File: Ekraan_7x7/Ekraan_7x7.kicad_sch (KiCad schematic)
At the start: 37 parts, among them IC1 74HC595PW-Q100,118, IC10 1EDN7550BXTSA1, IC11 1EDN7550BXTSA1, IC3 1EDN7550BXTSA1, IC6 1EDN7550BXTSA1, IC7 1EDN7550BXTSA1, IC8 1EDN7550BXTSA1, IC9 1EDN7550BXTSA1, U1 1EDN7550BXTSA1

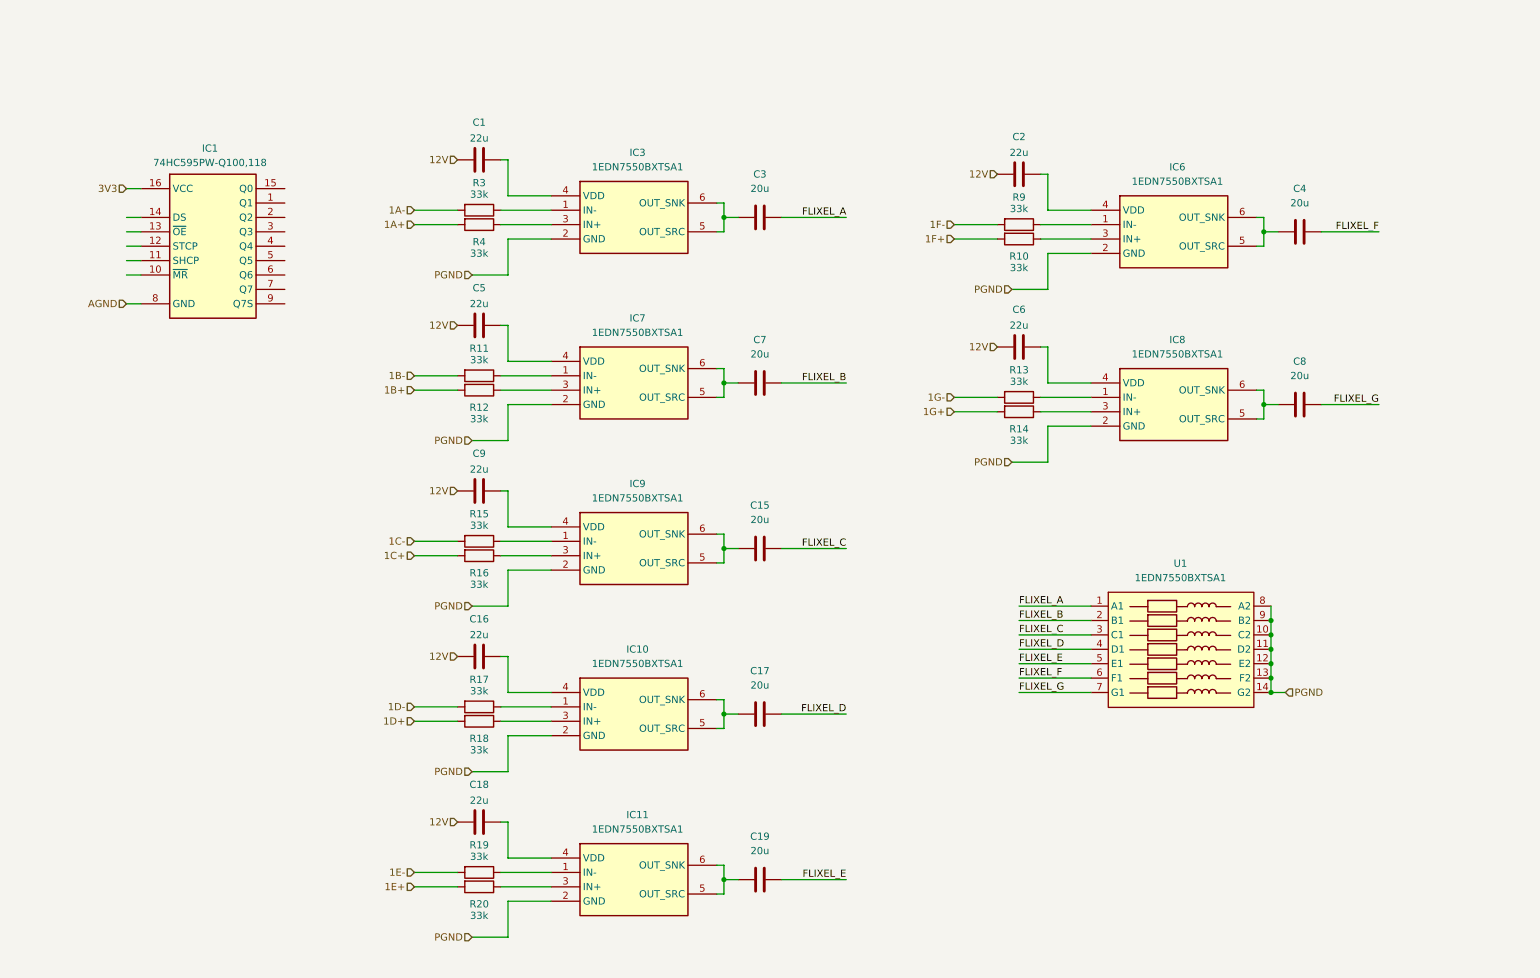
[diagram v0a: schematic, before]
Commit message: qqwertrewasdfgfdsdfgfdsdfgfdsasdfghgfdsdfghgfdsasdfghgfdsasdfgfew3
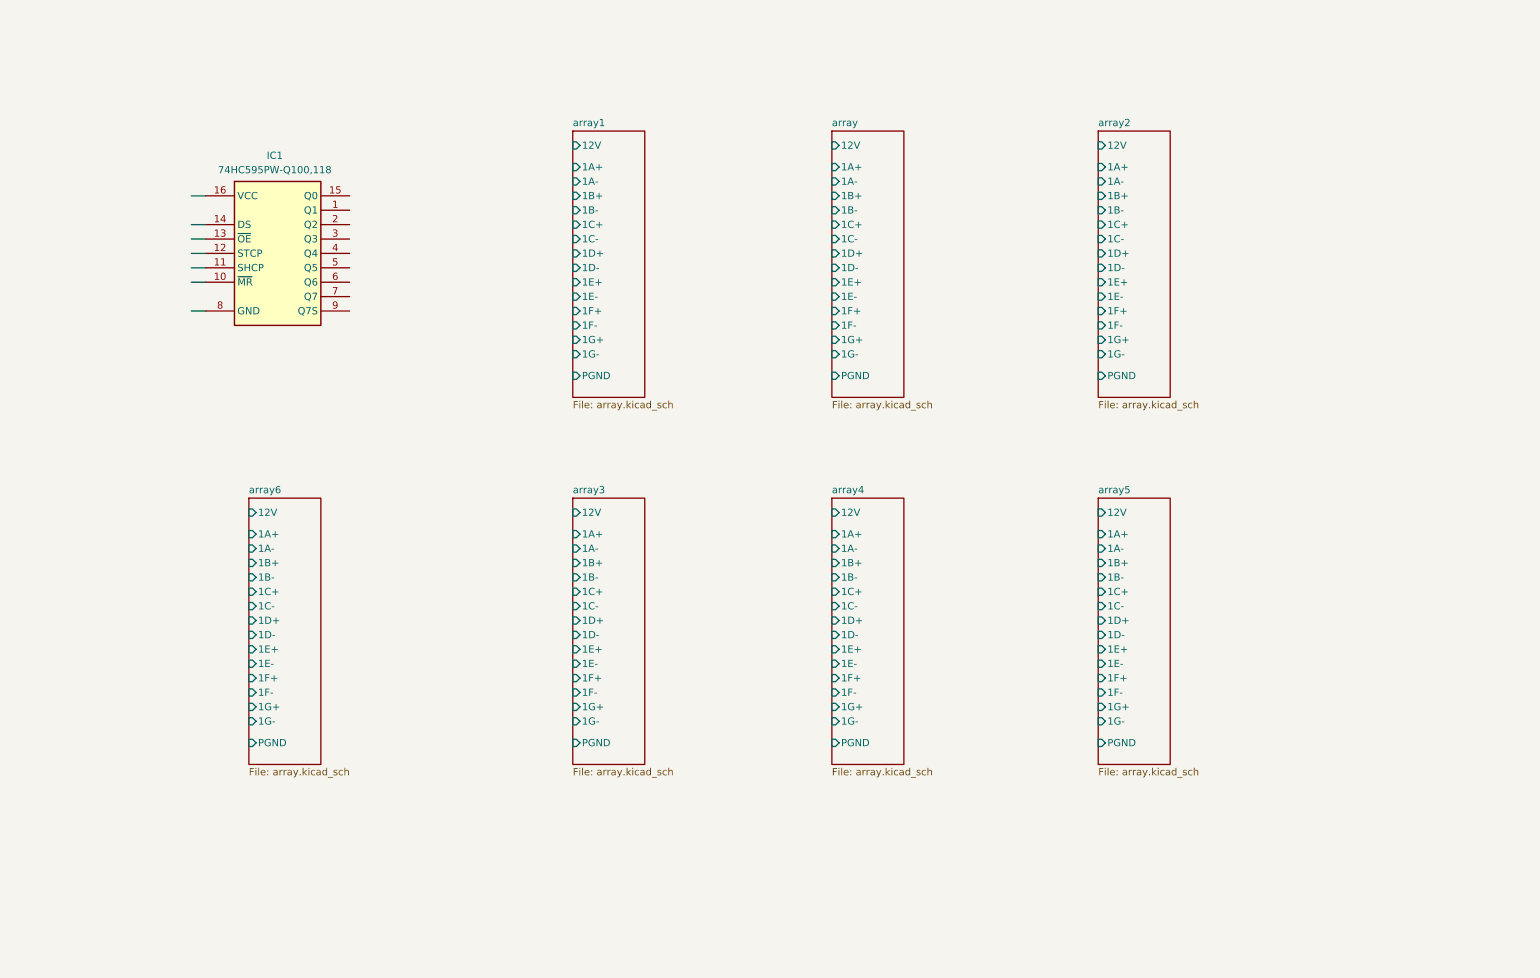
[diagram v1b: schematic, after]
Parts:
- removed C1, C16, C18, C2, C5, C6, C9: 22u, symbol Device:C
- removed C15, C17, C19, C3, C4, C7, C8: 20u, Capacitor_SMD:C_0201_0603Metric, symbol Device:C
- removed IC10, IC11, IC3, IC6, IC7, IC8, IC9: 1EDN7550BXTSA1, SOT95P280X145-6N, symbol 1EDN7550BXTSA1:1EDN7550BXTSA1
- removed R10, R11, R12, R13, R14, R15, R16, R17, R18, R19, R20, R3, R4, R9: 33k, symbol Device:R
- removed U1: 1EDN7550BXTSA1, dot_flipper:7_flip_dots, symbol flipdot_7xarray:flipdot_7xarray
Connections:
- net 3V3: no longer names the net of IC1.16 (VCC)
- net AGND: no longer names the net of IC1.8 (GND)
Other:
- added sheet array (array.kicad_sch)
- added sheet array1 (array.kicad_sch)
- added sheet array2 (array.kicad_sch)
- added sheet array3 (array.kicad_sch)
- added sheet array4 (array.kicad_sch)
- added sheet array5 (array.kicad_sch)
- added sheet array6 (array.kicad_sch)
- moved on the sheet: IC1

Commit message: Getamine addiction
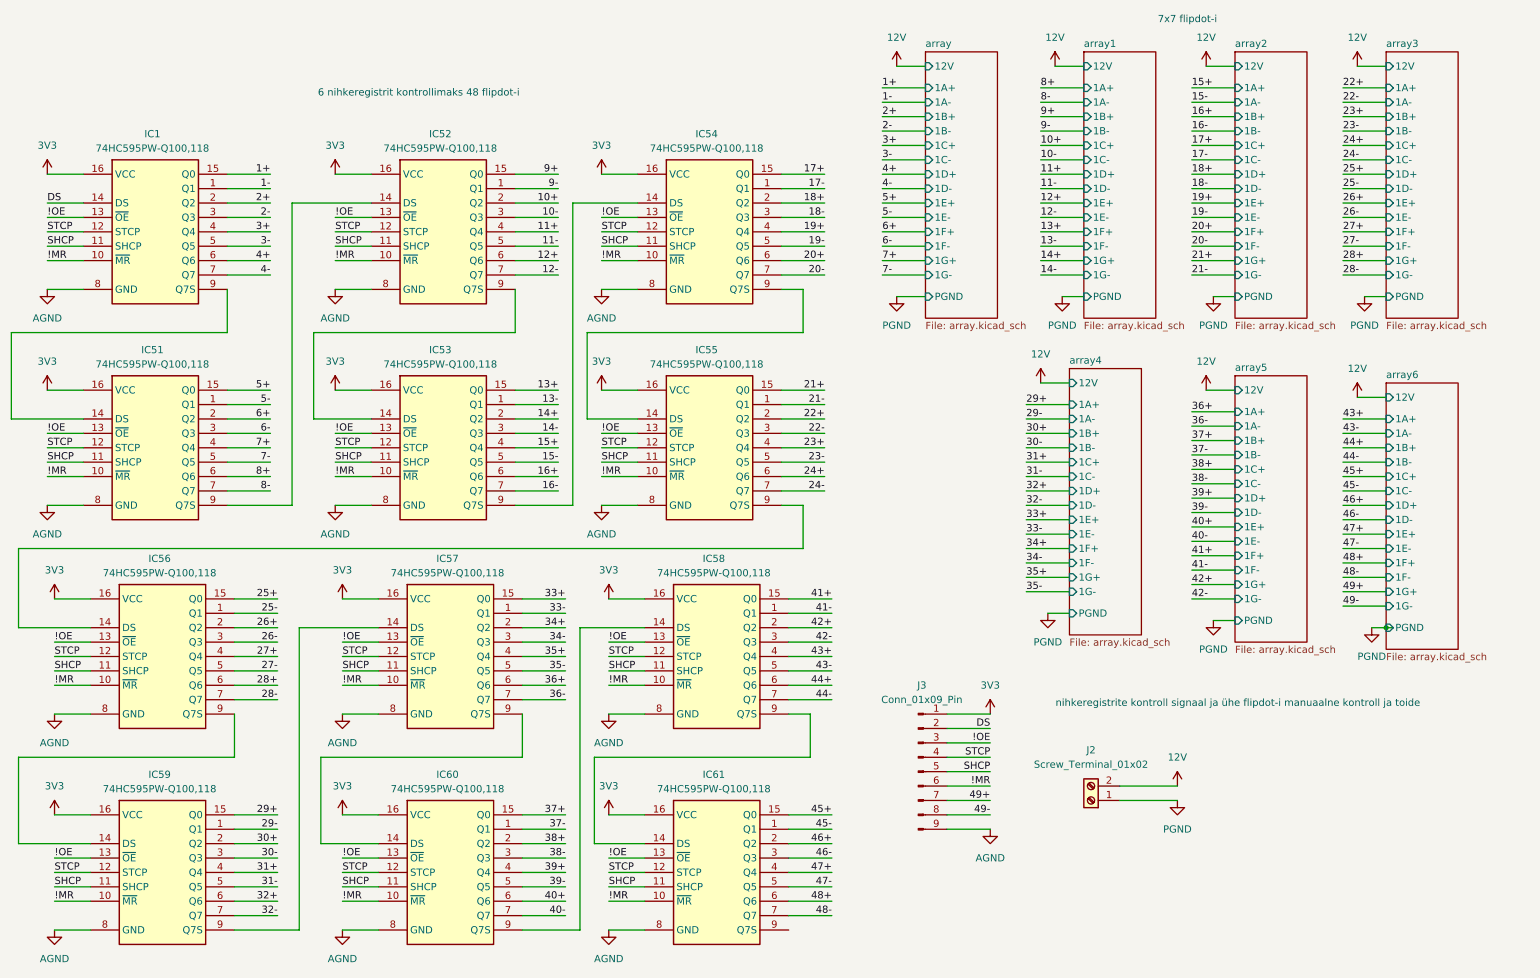
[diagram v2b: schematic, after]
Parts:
- added IC51, IC52, IC53, IC54, IC55, IC56, IC57, IC58, IC59, IC60, IC61: 74HC595PW-Q100,118, SOP65P640X110-16N, symbol 74HC595PW-Q100_118:74HC595PW-Q100,118
- added J2: Screw_Terminal_01x02, symbol Connector:Screw_Terminal_01x02
- added J3: Conn_01x09_Pin, symbol Connector:Conn_01x09_Pin
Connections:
- net 1-: now reaches IC1.1 (Q1)
- net !MR: now reaches IC1.10 (~{MR})
- net !MR: now also IC51.10 (~{MR}), IC52.10 (~{MR}), IC53.10 (~{MR}), IC54.10 (~{MR}), IC55.10 (~{MR}), IC56.10 (~{MR}), IC57.10 (~{MR}), IC58.10 (~{MR}), IC59.10 (~{MR}), IC60.10 (~{MR}), IC61.10 (~{MR}), J3.6 (Pin_6)
- net SHCP: now reaches IC1.11 (SHCP)
- net SHCP: now also IC51.11 (SHCP), IC52.11 (SHCP), IC53.11 (SHCP), IC54.11 (SHCP), IC55.11 (SHCP), IC56.11 (SHCP), IC57.11 (SHCP), IC58.11 (SHCP), IC59.11 (SHCP), IC60.11 (SHCP), IC61.11 (SHCP), J3.5 (Pin_5)
- net STCP: now reaches IC1.12 (STCP)
- net STCP: now also IC51.12 (STCP), IC52.12 (STCP), IC53.12 (STCP), IC54.12 (STCP), IC55.12 (STCP), IC56.12 (STCP), IC57.12 (STCP), IC58.12 (STCP), IC59.12 (STCP), IC60.12 (STCP), IC61.12 (STCP), J3.4 (Pin_4)
- net !OE: now reaches IC1.13 (~{OE})
- net !OE: now also IC51.13 (~{OE}), IC52.13 (~{OE}), IC53.13 (~{OE}), IC54.13 (~{OE}), IC55.13 (~{OE}), IC56.13 (~{OE}), IC57.13 (~{OE}), IC58.13 (~{OE}), IC59.13 (~{OE}), IC60.13 (~{OE}), IC61.13 (~{OE}), J3.3 (Pin_3)
- net DS: now reaches IC1.14 (DS)
- net DS: now also J3.2 (Pin_2)
- net 1+: now reaches IC1.15 (Q0)
- net 3V3: now reaches IC1.16 (VCC)
- net 3V3: now also IC51.16 (VCC), IC52.16 (VCC), IC53.16 (VCC), IC54.16 (VCC), IC55.16 (VCC), IC56.16 (VCC), IC57.16 (VCC), IC58.16 (VCC), IC59.16 (VCC), IC60.16 (VCC), IC61.16 (VCC), J3.1 (Pin_1)
- net 2+: now reaches IC1.2 (Q2)
- net 2-: now reaches IC1.3 (Q3)
- net 3+: now reaches IC1.4 (Q4)
- net 3-: now reaches IC1.5 (Q5)
- net 4+: now reaches IC1.6 (Q6)
- net 4-: now reaches IC1.7 (Q7)
- net AGND: now reaches IC1.8 (GND)
- net AGND: now also IC51.8 (GND), IC52.8 (GND), IC53.8 (GND), IC54.8 (GND), IC55.8 (GND), IC56.8 (GND), IC57.8 (GND), IC58.8 (GND), IC59.8 (GND), IC60.8 (GND), IC61.8 (GND), J3.9 (Pin_9)
- net at IC1.9 (Q7S): now also IC51.14 (DS)
- new net: IC57.14 (DS), IC59.9 (Q7S)
- new net: IC57.9 (Q7S), IC60.14 (DS)
- new net: IC55.9 (Q7S), IC56.14 (DS)
- new net: IC56.9 (Q7S), IC59.14 (DS)
- new net: IC51.9 (Q7S), IC52.14 (DS)
- new net: IC52.9 (Q7S), IC53.14 (DS)
- new net: IC58.14 (DS), IC60.9 (Q7S)
- new net: IC58.9 (Q7S), IC61.14 (DS)
- new net: IC53.9 (Q7S), IC54.14 (DS)
- new net: IC54.9 (Q7S), IC55.14 (DS)
- new net 10+: IC52.2 (Q2)
- new net 10-: IC52.3 (Q3)
- new net 11+: IC52.4 (Q4)
- new net 11-: IC52.5 (Q5)
- new net 12+: IC52.6 (Q6)
- new net 12-: IC52.7 (Q7)
- new net 12V: J2.2 (Pin_2)
- new net 13+: IC53.15 (Q0)
- new net 13-: IC53.1 (Q1)
- new net 14+: IC53.2 (Q2)
- new net 14-: IC53.3 (Q3)
- new net 15+: IC53.4 (Q4)
- new net 15-: IC53.5 (Q5)
- new net 16+: IC53.6 (Q6)
- new net 16-: IC53.7 (Q7)
- new net 17+: IC54.15 (Q0)
- new net 17-: IC54.1 (Q1)
- new net 18+: IC54.2 (Q2)
- new net 18-: IC54.3 (Q3)
- new net 19+: IC54.4 (Q4)
- new net 19-: IC54.5 (Q5)
- new net 20+: IC54.6 (Q6)
- new net 20-: IC54.7 (Q7)
- new net 21+: IC55.15 (Q0)
- new net 21-: IC55.1 (Q1)
- new net 22+: IC55.2 (Q2)
- new net 22-: IC55.3 (Q3)
- new net 23+: IC55.4 (Q4)
- new net 23-: IC55.5 (Q5)
- new net 24+: IC55.6 (Q6)
- new net 24-: IC55.7 (Q7)
- new net 25+: IC56.15 (Q0)
- new net 25-: IC56.1 (Q1)
- new net 26+: IC56.2 (Q2)
- new net 26-: IC56.3 (Q3)
- new net 27+: IC56.4 (Q4)
- new net 27-: IC56.5 (Q5)
- new net 28+: IC56.6 (Q6)
- new net 28-: IC56.7 (Q7)
- new net 29+: IC59.15 (Q0)
- new net 29-: IC59.1 (Q1)
- new net 30+: IC59.2 (Q2)
- new net 30-: IC59.3 (Q3)
- new net 31+: IC59.4 (Q4)
- new net 31-: IC59.5 (Q5)
- new net 32+: IC59.6 (Q6)
- new net 32-: IC59.7 (Q7)
- new net 33+: IC57.15 (Q0)
- new net 33-: IC57.1 (Q1)
- new net 34+: IC57.2 (Q2)
- new net 34-: IC57.3 (Q3)
- new net 35+: IC57.4 (Q4)
- new net 35-: IC57.5 (Q5)
- new net 36+: IC57.6 (Q6)
- new net 36-: IC57.7 (Q7)
- new net 37+: IC60.15 (Q0)
- new net 37-: IC60.1 (Q1)
- new net 38+: IC60.2 (Q2)
- new net 38-: IC60.3 (Q3)
- new net 39+: IC60.4 (Q4)
- new net 39-: IC60.5 (Q5)
- new net 40+: IC60.6 (Q6)
- new net 40-: IC60.7 (Q7)
- new net 41+: IC58.15 (Q0)
- new net 41-: IC58.1 (Q1)
- new net 42+: IC58.2 (Q2)
- new net 42-: IC58.3 (Q3)
- new net 43+: IC58.4 (Q4)
- new net 43-: IC58.5 (Q5)
- new net 44+: IC58.6 (Q6)
- new net 44-: IC58.7 (Q7)
- new net 45+: IC61.15 (Q0)
- new net 45-: IC61.1 (Q1)
- new net 46+: IC61.2 (Q2)
- new net 46-: IC61.3 (Q3)
- new net 47+: IC61.4 (Q4)
- new net 47-: IC61.5 (Q5)
- new net 48+: IC61.6 (Q6)
- new net 48-: IC61.7 (Q7)
- new net 49+: J3.7 (Pin_7)
- new net 49-: J3.8 (Pin_8)
- new net 5+: IC51.15 (Q0)
- new net 5-: IC51.1 (Q1)
- new net 6+: IC51.2 (Q2)
- new net 6-: IC51.3 (Q3)
- new net 7+: IC51.4 (Q4)
- new net 7-: IC51.5 (Q5)
- new net 8+: IC51.6 (Q6)
- new net 8-: IC51.7 (Q7)
- new net 9+: IC52.15 (Q0)
- new net 9-: IC52.1 (Q1)
- new net PGND: J2.1 (Pin_1)
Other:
- note added: "6 nihkeregistrit kontrollimaks 48 flipdot-i"
- note added: "7x7 flipdot-i"
- note added: "nihkeregistrite kontroll signaal ja ühe flipdot-i manuaalne kontroll ja toide"
- moved on the sheet: IC1
